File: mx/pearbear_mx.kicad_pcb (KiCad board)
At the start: 2 copper layers, 122.7 x 76.2 mm, 26 parts, among them J1 rj11, SW1 SW_Push, SW10 SW_Push, SW11 SW_Push, SW12 SW_Push, SW13 SW_Push, SW14 SW_Push, SW15 SW_Push, SW16 SW_Push, SW17 SW_Push, SW2 SW_Push, SW3 SW_Push, SW4 SW_Push, SW5 SW_Push, SW6 SW_Push, SW7 SW_Push, SW8 SW_Push, SW9 SW_Push, U1 ProMicro-kbd-rev

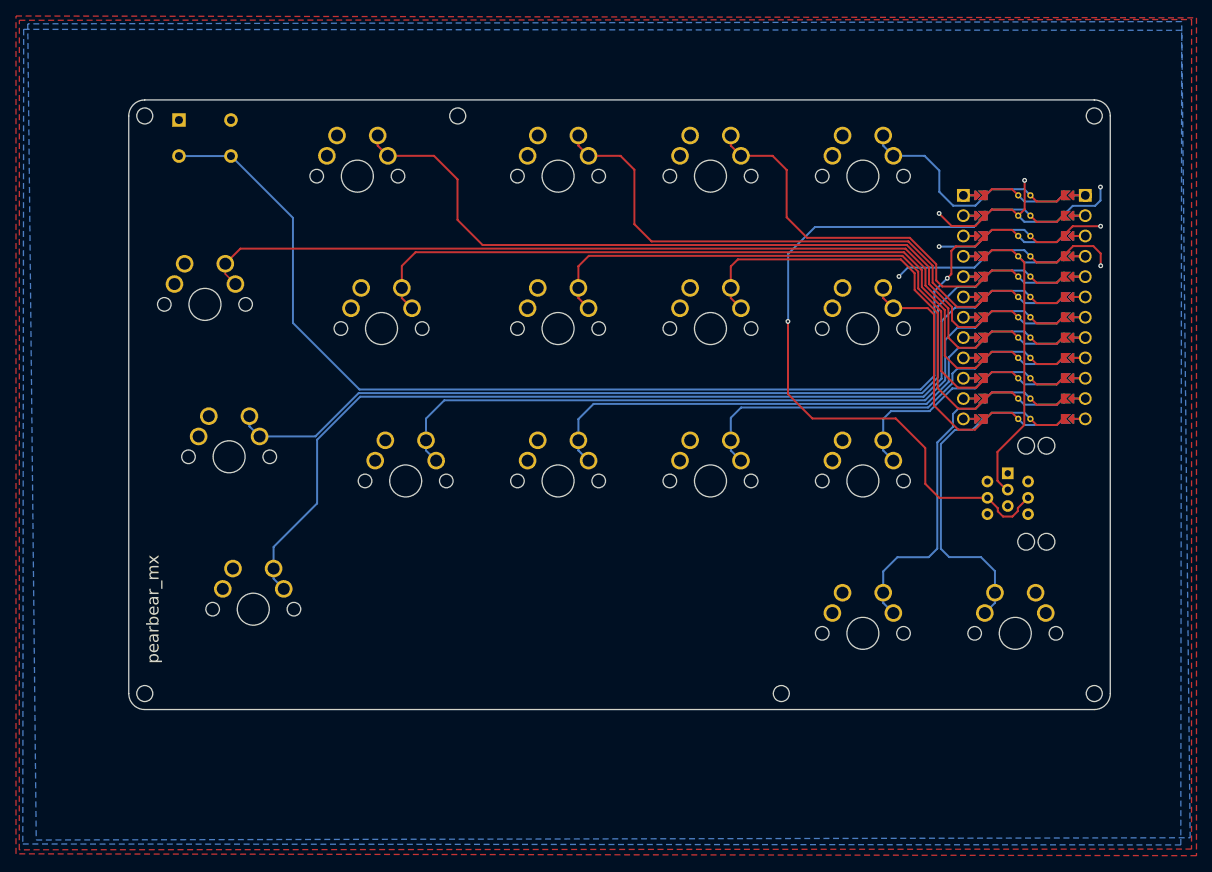
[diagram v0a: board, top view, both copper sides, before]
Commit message: hi
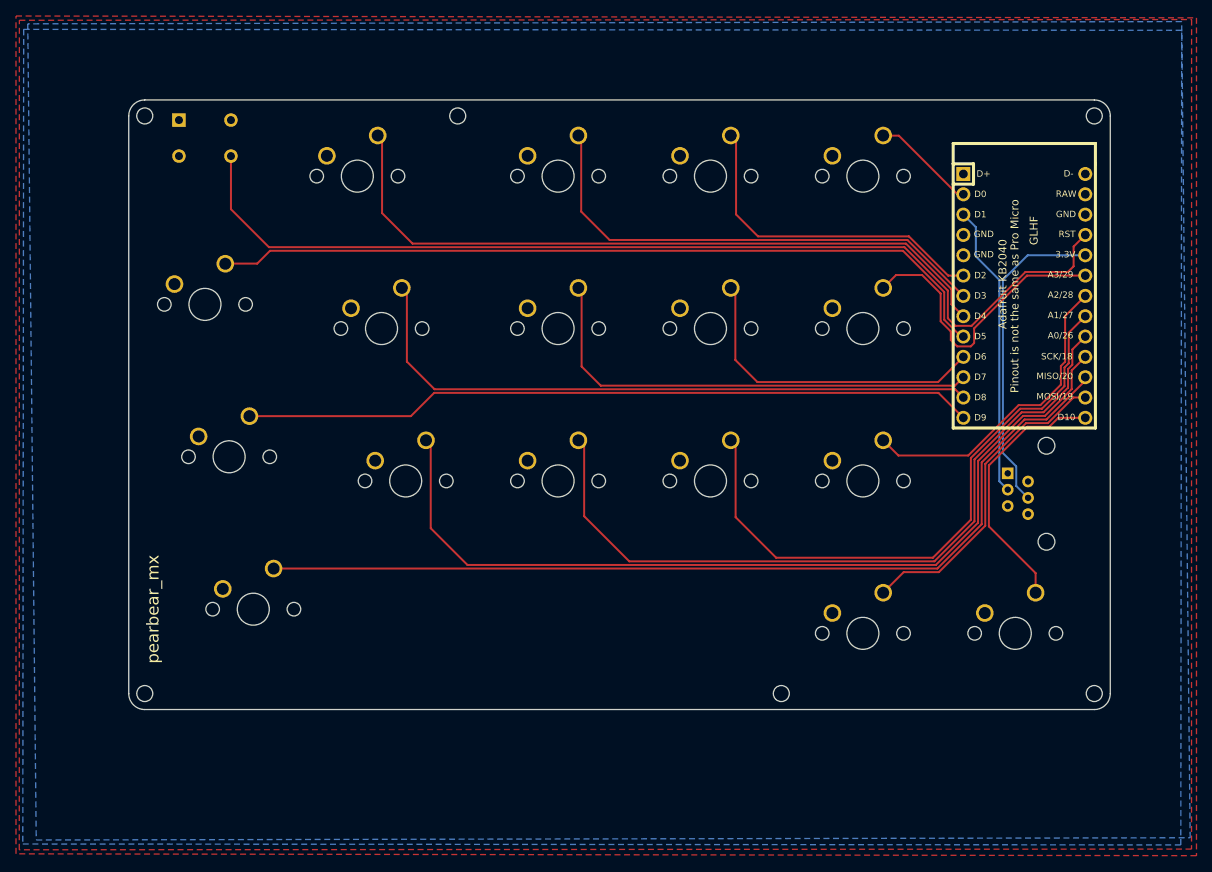
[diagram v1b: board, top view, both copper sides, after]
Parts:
- J1: footprint pb_fp:RJ11_6P6C_reversible -> pb_fp:RJ11_6P6C
- SW1, SW10, SW11, SW12, SW13, SW14, SW15, SW16, SW2, SW3, SW4, SW5, SW6, SW7, SW8, SW9: footprint pb_fp:SW_Cherry_MX_reversible -> pb_fp:SW_Cherry_MX
- SW17: footprint pb_fp:SW_Cherry_MX_reversible -> pb_fp:SW_Cherry_MX; moved to F.Cu
- U1: footprint pb_fp:ProMicro_reversible -> pb_fp:kb2040
- moved U1 2.67 mm to (201.5, 82.5), turned to 0 degrees
- turned SW17 to 0 degrees
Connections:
- J1 pad 3: vcc -> rjdata
- J1 pad 4: rjdata -> vcc
- U1 pad 10: Switch8 -> Switch11
- U1 pad 11: Switch9 -> Switch16
- U1 pad 12: Switch10 -> Switch17
- U1 pad 13: Switch17 -> Switch6
- U1 pad 14: Switch16 -> Switch7
- U1 pad 15: Switch15 -> Switch8
- U1 pad 16: Switch14 -> Switch9
- U1 pad 17: Switch13 -> Switch1
- U1 pad 18: Switch12 -> Switch2
- U1 pad 19: Switch11 -> Switch3
- U1 pad 20: Switch6 -> Switch4
- U1 pad 5: Switch4 -> Switch10
- U1 pad 6: Switch3 -> Switch15
- U1 pad 7: Switch2 -> Switch14
- U1 pad 8: Switch1 -> Switch13
- U1 pad 9: Switch7 -> Switch12
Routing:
- net gnd: track 49.6 -> 0.00 mm, vias 7 -> 0
- net rjdata: track 84.6 -> 36.7 mm, vias 1 -> 0
- net Switch14: track 41.5 -> 76.3 mm
- net Switch13: track 62.6 -> 93.4 mm
- net Switch12: track 83.9 -> 111.6 mm
- net Switch15: track 20.7 -> 39.0 mm
- net Switch6: track 107.3 -> 91.7 mm
- net Switch9: track 52.9 -> 40.2 mm
- net Switch8: track 70.1 -> 59.1 mm
- net Switch7: track 90.6 -> 80.9 mm
- net Switch10: track 28.1 -> 37.0 mm
- net reset: track 136.5 -> 127.6 mm, vias 1 -> 0
- net vcc: track 31.5 -> 40.1 mm
- net Switch1: track 107.9 -> 99.4 mm
- net Switch5: track 19.3 -> 13.1 mm
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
